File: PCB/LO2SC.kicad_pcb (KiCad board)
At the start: 2 copper layers, 6 parts, among them U1 TLV2252AID

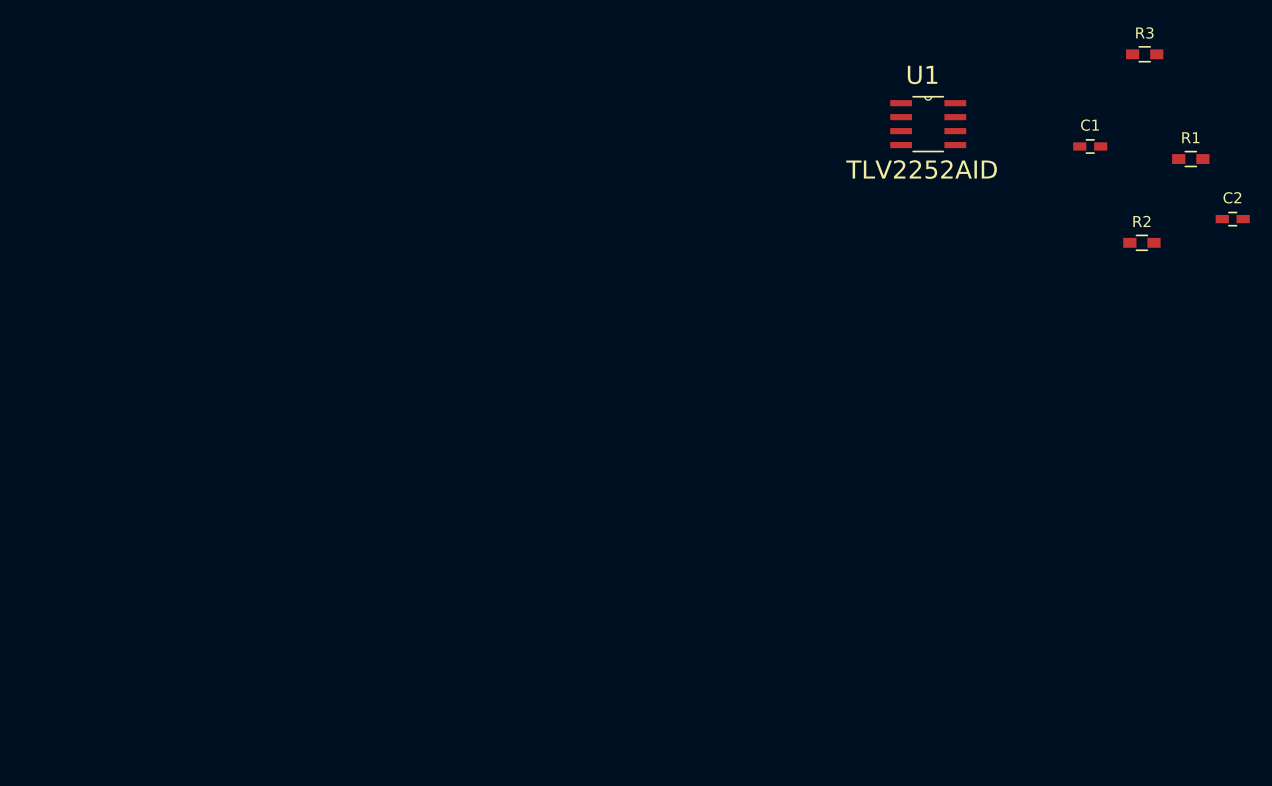
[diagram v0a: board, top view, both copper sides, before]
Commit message: - ajout de schematiques
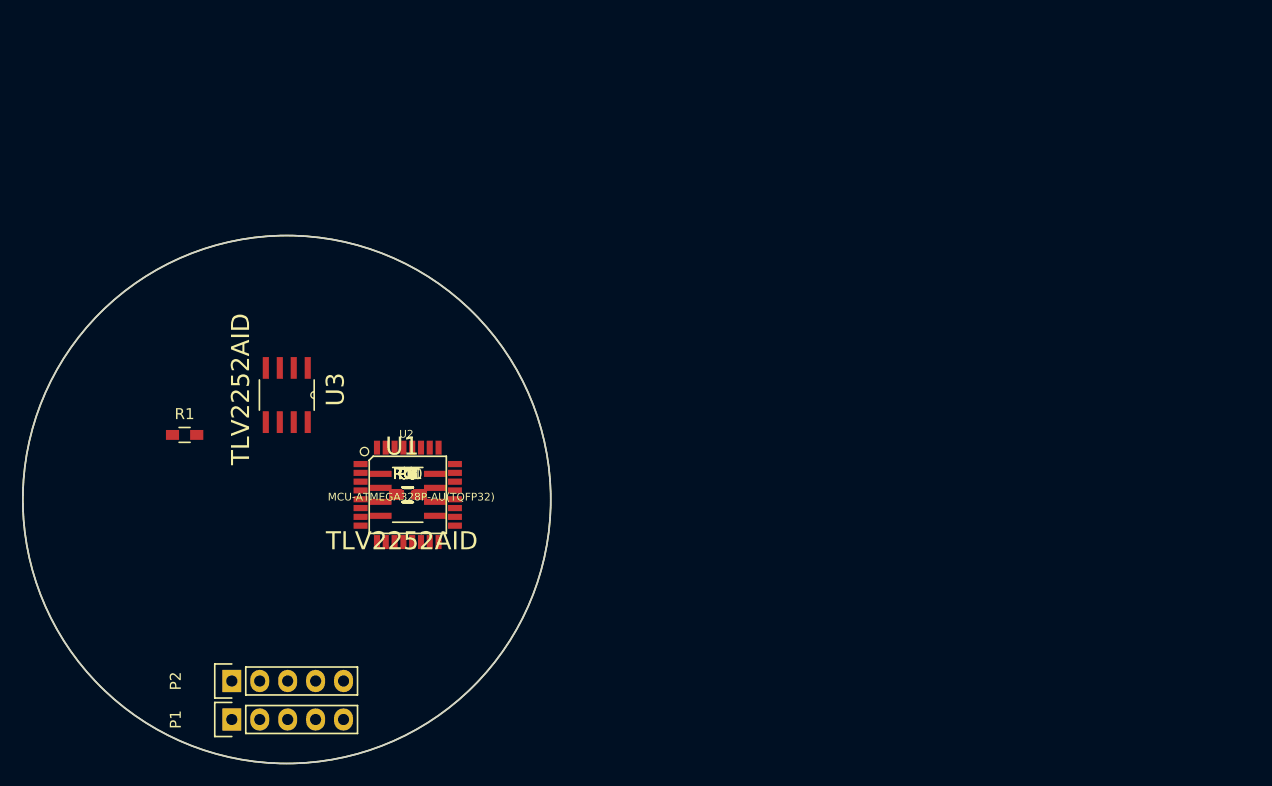
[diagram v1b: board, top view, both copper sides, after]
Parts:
- added C3: 10nF, condensateurs:C_0603_HandSoldering, F.Cu at (92.0, 120.6)
- added C4: 100nF, condensateurs:C_0603_HandSoldering, F.Cu at (92.0, 120.6)
- added P1: CONN_01X05, Barrettes:Pin_Header_Straight_1x05, F.Cu at (76.0, 141.0)
- added P2: CONN_01X05, Barrettes:Pin_Header_Straight_1x05, F.Cu at (76.0, 137.5)
- added R10, R11, R9: 10k, resistances:R_0603_HandSoldering, F.Cu at (92.0, 120.6)
- added R4: 470k, resistances:R_0603_HandSoldering, F.Cu at (92.0, 120.6)
- added R5: 22k, resistances:R_0603_HandSoldering, F.Cu at (92.0, 120.6)
- added R6: 330k, resistances:R_0603_HandSoldering, F.Cu at (92.0, 120.6)
- added R7: 62, resistances:R_0603_HandSoldering, F.Cu at (92.0, 120.6)
- added R8: 47k, resistances:R_0603_HandSoldering, F.Cu at (92.0, 120.6)
- added Ref**: Val**, PCB:vue3D, F.Cu at (81.0, 121.0)
- added U2: MCU-ATMEGA328P-AU(TQFP32), atmel:TQFP32-0.8-7X7MM, F.Cu at (92.0, 120.6)
- added U3: TLV2252AID, Amplificateur_Operationel:SOIC127P600X175-8N, F.Cu at (81.0, 111.5)
- moved R1 94.9 mm to (71.7, 115.1)
- moved C2 79.1 mm to (92.0, 120.6)
- moved R3 78.1 mm to (92.0, 120.6)
- moved R2 70.6 mm to (92.0, 120.6)
- moved C1 69.7 mm to (92.0, 120.6)
- moved U1 58.1 mm to (92.0, 120.6)
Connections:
- net OUT1 renamed 2.5v
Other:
- board outline added: 48 x 48 mm
- net class Default: clearance 0.2 -> 0.25
- rule trace_clearance: 0.2 -> 0.25
- rule trace_min: 0.2 -> 0.25
